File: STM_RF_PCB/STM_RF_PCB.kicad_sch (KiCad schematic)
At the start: 48 parts, among them J1 SMA, J2 USB_B_Micro, J3 SWD STLINk, J4 Conn_01x04, SW1 UP, SW2 LF, SW3 DN, SW4 RT, SW5 A, SW6 B, SW7 SELECT, SW8 START, U1 nRF24L01P, U2 USBLC6-2SC6, U3 XC6206P332MR, U4 STM32L432KBUx, Y1 16 MHz

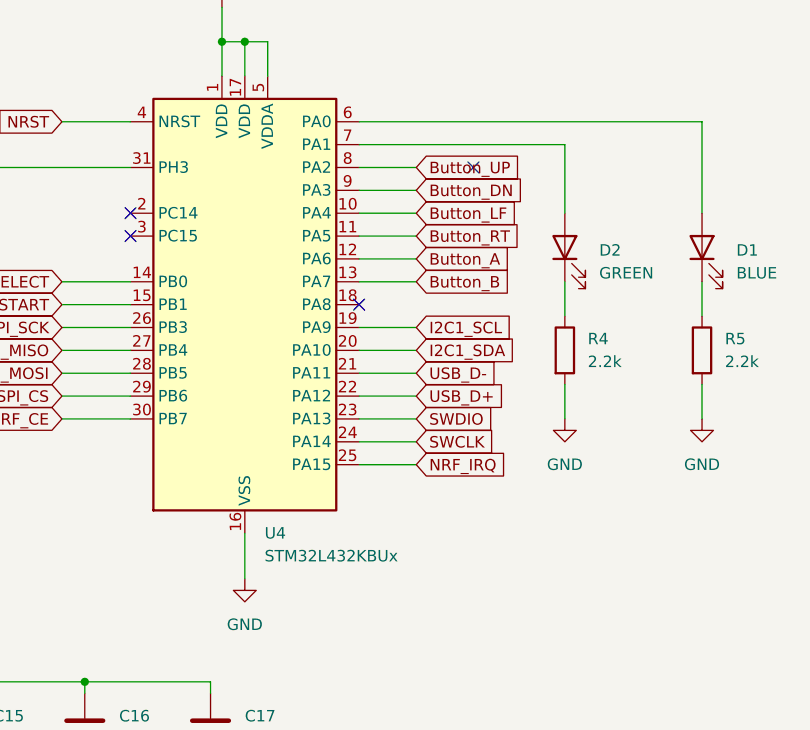
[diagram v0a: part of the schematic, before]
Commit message: PCB work
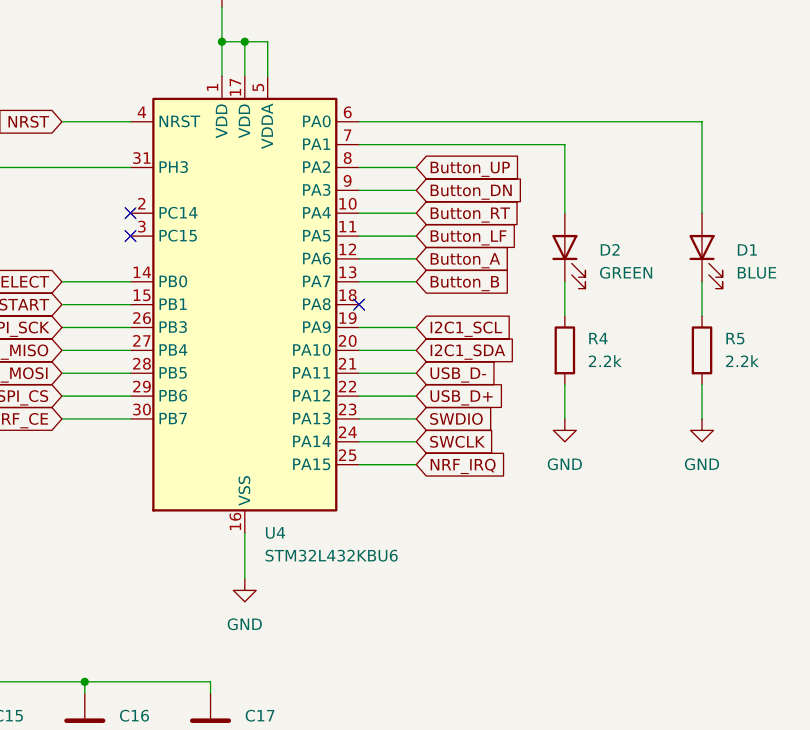
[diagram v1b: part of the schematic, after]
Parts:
- U3: footprint Package_TO_SOT_SMD:SOT-23-3 -> Library:XC6206P332MR
- U4: value STM32L432KBUx -> STM32L432KBU6; footprint Package_DFN_QFN:UFQFPN-32-1EP_5x5mm_P0.5mm_EP3.5x3.5mm -> Library:STM32L432KBU6
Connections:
- net Button_LF: now also U4.11 (PA5); no longer U4.10 (PA4)
- net Button_RT: now also U4.10 (PA4); no longer U4.11 (PA5)
- no-connect marks 9 -> 8
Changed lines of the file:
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@@
 	)
 	(no_connect
-		(at 342.9 161.29)
-	)
-	(no_connect
 		(at 283.21 116.84)
 	)
@@
 	(wire
 		(pts
+			(xy 330.2 168.91) (xy 336.55 168.91)
+		)
+		(stroke
+			(width 0)
+			(type default)
+		)
+	)
+	(wire
+		(pts
 			(xy 66.04 170.18) (xy 66.04 166.37)
 		)
@@
 	(wire
 		(pts
-			(xy 330.2 166.37) (xy 336.55 166.37)
-		)
-		(stroke
-			(width 0)
-			(type default)
-		)
-	)
-	(wire
-		(pts
 			(xy 330.2 171.45) (xy 336.55 171.45)
 		)
@@
 	(wire
 		(pts
+			(xy 330.2 166.37) (xy 336.55 166.37)
+		)
+		(stroke
+			(width 0)
+			(type default)
+		)
+	)
+	(wire
+		(pts
 			(xy 110.49 215.9) (xy 110.49 209.55)
 		)
@@
 	(wire
 		(pts
-			(xy 330.2 168.91) (xy 336.55 168.91)
-		)
-		(stroke
-			(width 0)
-			(type default)
-		)
-	)
-	(wire
-		(pts
 			(xy 54.61 246.38) (xy 54.61 248.92)
 		)
@@
 	(global_label "Button_RT"
 		(shape input)
-		(at 336.55 168.91 0)
+		(at 336.55 166.37 0)
 		(fields_autoplaced yes)
 		(effects
@@
 		)
 		(property "Intersheetrefs" "${INTERSHEET_REFS}"
-			(at 348.9088 168.91 0)
+			(at 348.9088 166.37 0)
 			(effects
 				(font
@@
 	(global_label "Button_LF"
 		(shape input)
-		(at 336.55 166.37 0)
+		(at 336.55 168.91 0)
 		(fields_autoplaced yes)
 		(effects
@@
 		)
 		(property "Intersheetrefs" "${INTERSHEET_REFS}"
-			(at 348.7879 166.37 0)
+			(at 348.7879 168.91 0)
 			(effects
 				(font
@@
 			)
 		)
-		(property "Value" "STM32L432KBUx"
+		(property "Value" "STM32L432KBU6"
 			(at 319.6941 204.47 0)
 			(effects
@@
 			)
 		)
-		(property "Footprint" "Package_DFN_QFN:UFQFPN-32-1EP_5x5mm_P0.5mm_EP3.5x3.5mm"
+		(property "Footprint" "Library:STM32L432KBU6"
 			(at 307.34 199.39 0)
 			(effects
@@
 			)
 		)
-		(property "Footprint" "Package_TO_SOT_SMD:SOT-23-3"
+		(property "Footprint" "Library:XC6206P332MR"
 			(at 132.08 29.845 0)
 			(effects

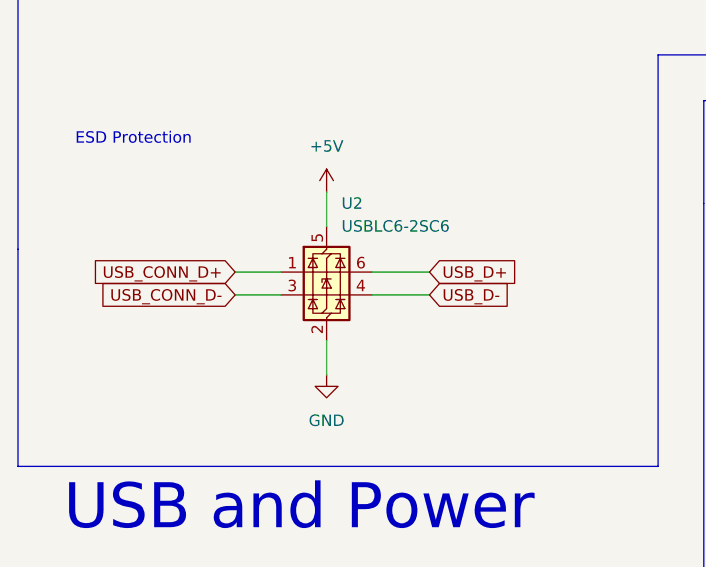
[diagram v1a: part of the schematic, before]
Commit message: pcb work
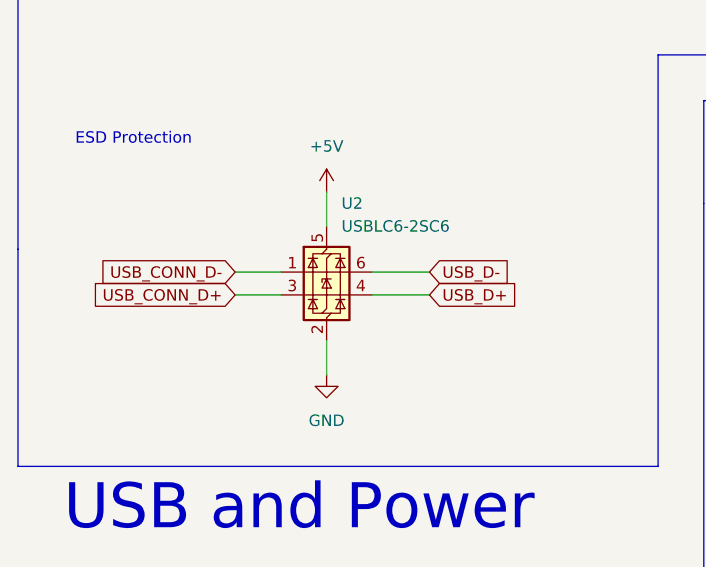
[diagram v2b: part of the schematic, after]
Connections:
- net USB_CONN_D+: now also U2.3 (I/O2); no longer U2.1 (I/O1)
- net USB_CONN_D-: now also U2.1 (I/O1); no longer U2.3 (I/O2)
- net USB_D+: now also U2.4 (I/O2); no longer U2.6 (I/O1)
- net USB_D-: now also U2.6 (I/O1); no longer U2.4 (I/O2)
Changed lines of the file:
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@@
 	(wire
 		(pts
+			(xy 52.07 91.44) (xy 58.42 91.44)
+		)
+		(stroke
+			(width 0)
+			(type default)
+		)
+	)
+	(wire
+		(pts
 			(xy 116.84 48.26) (xy 116.84 52.07)
 		)
@@
 	(wire
 		(pts
-			(xy 52.07 91.44) (xy 58.42 91.44)
-		)
-		(stroke
-			(width 0)
-			(type default)
-		)
-	)
-	(wire
-		(pts
 			(xy 54.61 237.49) (xy 43.18 237.49)
 		)
@@
 	(wire
 		(pts
+			(xy 36.83 93.98) (xy 41.91 93.98)
+		)
+		(stroke
+			(width 0)
+			(type default)
+		)
+	)
+	(wire
+		(pts
 			(xy 297.18 184.15) (xy 304.8 184.15)
 		)
@@
 	(wire
 		(pts
+			(xy 36.83 91.44) (xy 41.91 91.44)
+		)
+		(stroke
+			(width 0)
+			(type default)
+		)
+	)
+	(wire
+		(pts
 			(xy 330.2 168.91) (xy 336.55 168.91)
 		)
@@
 	(wire
 		(pts
-			(xy 342.9 101.6) (xy 342.9 99.06)
+			(xy 52.07 93.98) (xy 58.42 93.98)
 		)
 		(stroke
@@
 	(wire
 		(pts
-			(xy 314.96 147.32) (xy 314.96 151.13)
+			(xy 342.9 101.6) (xy 342.9 99.06)
 		)
 		(stroke
@@
 	(wire
 		(pts
-			(xy 36.83 91.44) (xy 41.91 91.44)
+			(xy 314.96 147.32) (xy 314.96 151.13)
 		)
 		(stroke
@@
 		)
 	)
-	(wire
-		(pts
-			(xy 52.07 93.98) (xy 58.42 93.98)
-		)
-		(stroke
-			(width 0)
-			(type default)
-		)
-	)
 	(polyline
 		(pts
@@
 	(wire
 		(pts
-			(xy 36.83 93.98) (xy 41.91 93.98)
-		)
-		(stroke
-			(width 0)
-			(type default)
-		)
-	)
-	(wire
-		(pts
 			(xy 349.25 36.83) (xy 355.6 36.83)
 		)
@@
 	(global_label "USB_D-"
 		(shape input)
-		(at 58.42 93.98 0)
+		(at 58.42 91.44 0)
 		(fields_autoplaced yes)
 		(effects
@@
 		)
 		(property "Intersheetrefs" "${INTERSHEET_REFS}"
-			(at 69.0252 93.98 0)
+			(at 69.0252 91.44 0)
 			(effects
 				(font
@@
 	(global_label "USB_CONN_D-"
 		(shape input)
-		(at 36.83 93.98 180)
+		(at 36.83 91.44 180)
 		(fields_autoplaced yes)
 		(effects
@@
 		)
 		(property "Intersheetrefs" "${INTERSHEET_REFS}"
-			(at 19.9957 93.98 0)
+			(at 19.9957 91.44 0)
 			(effects
 				(font
@@
 	(global_label "USB_D+"
 		(shape input)
-		(at 58.42 91.44 0)
+		(at 58.42 93.98 0)
 		(fields_autoplaced yes)
 		(effects
@@
 		)
 		(property "Intersheetrefs" "${INTERSHEET_REFS}"
-			(at 69.0252 91.44 0)
+			(at 69.0252 93.98 0)
 			(effects
 				(font
@@
 	(global_label "USB_CONN_D+"
 		(shape input)
-		(at 36.83 91.44 180)
+		(at 36.83 93.98 180)
 		(fields_autoplaced yes)
 		(effects
@@
 		)
 		(property "Intersheetrefs" "${INTERSHEET_REFS}"
-			(at 19.9957 91.44 0)
+			(at 19.9957 93.98 0)
 			(effects
 				(font

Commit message: Fab outputs
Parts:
- C2: Part ID CL10A106KP8NNNC -> 0603B103K101NT
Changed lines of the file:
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@@
 			)
 		)
-		(property "Part ID" "CL10A106KP8NNNC"
+		(property "Part ID" "0603B103K101NT"
 			(at 31.75 242.57 0)
 			(effects
